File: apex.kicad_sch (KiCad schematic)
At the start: 15 parts, among them J1 USB_C_Receptacle_USB2.0_16P, U1 AP7363-33D-13, U2 USBLC6-2P6

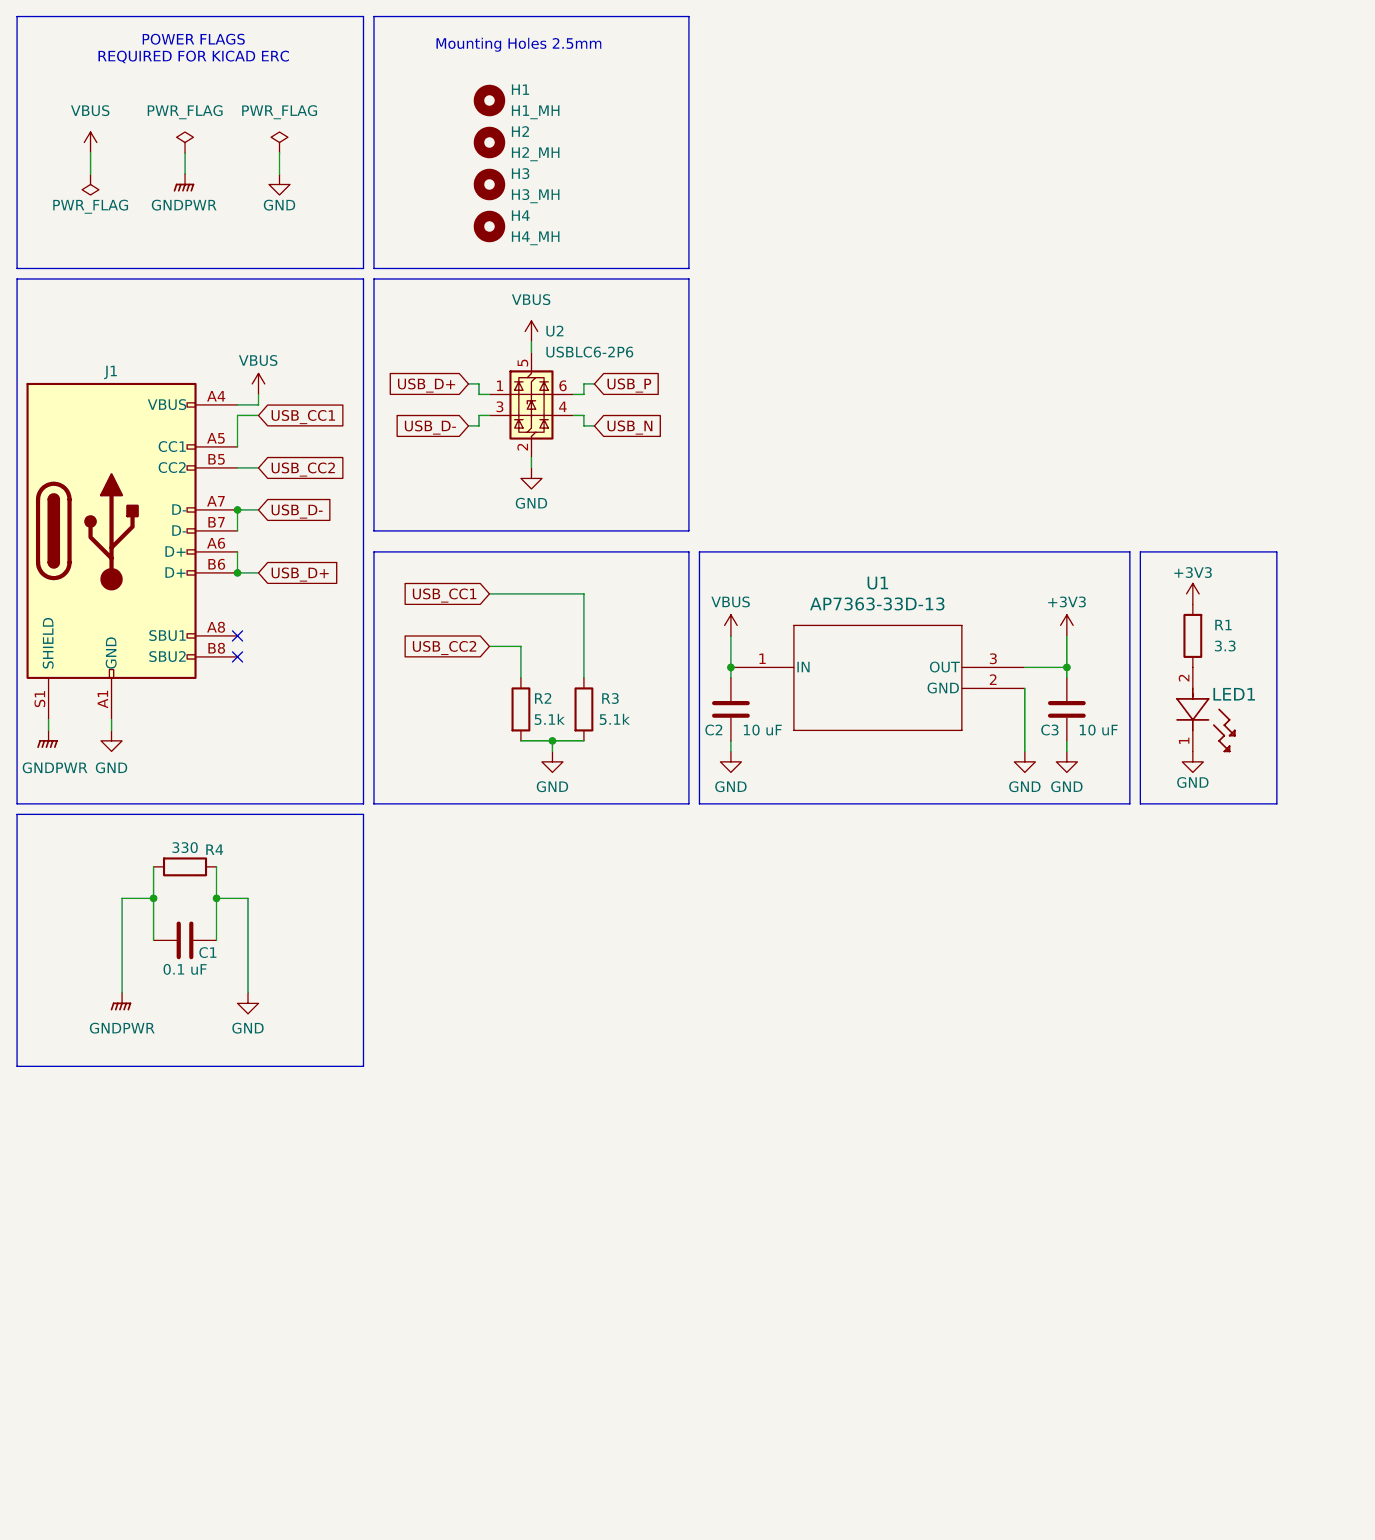
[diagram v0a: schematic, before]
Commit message: re-added symbols
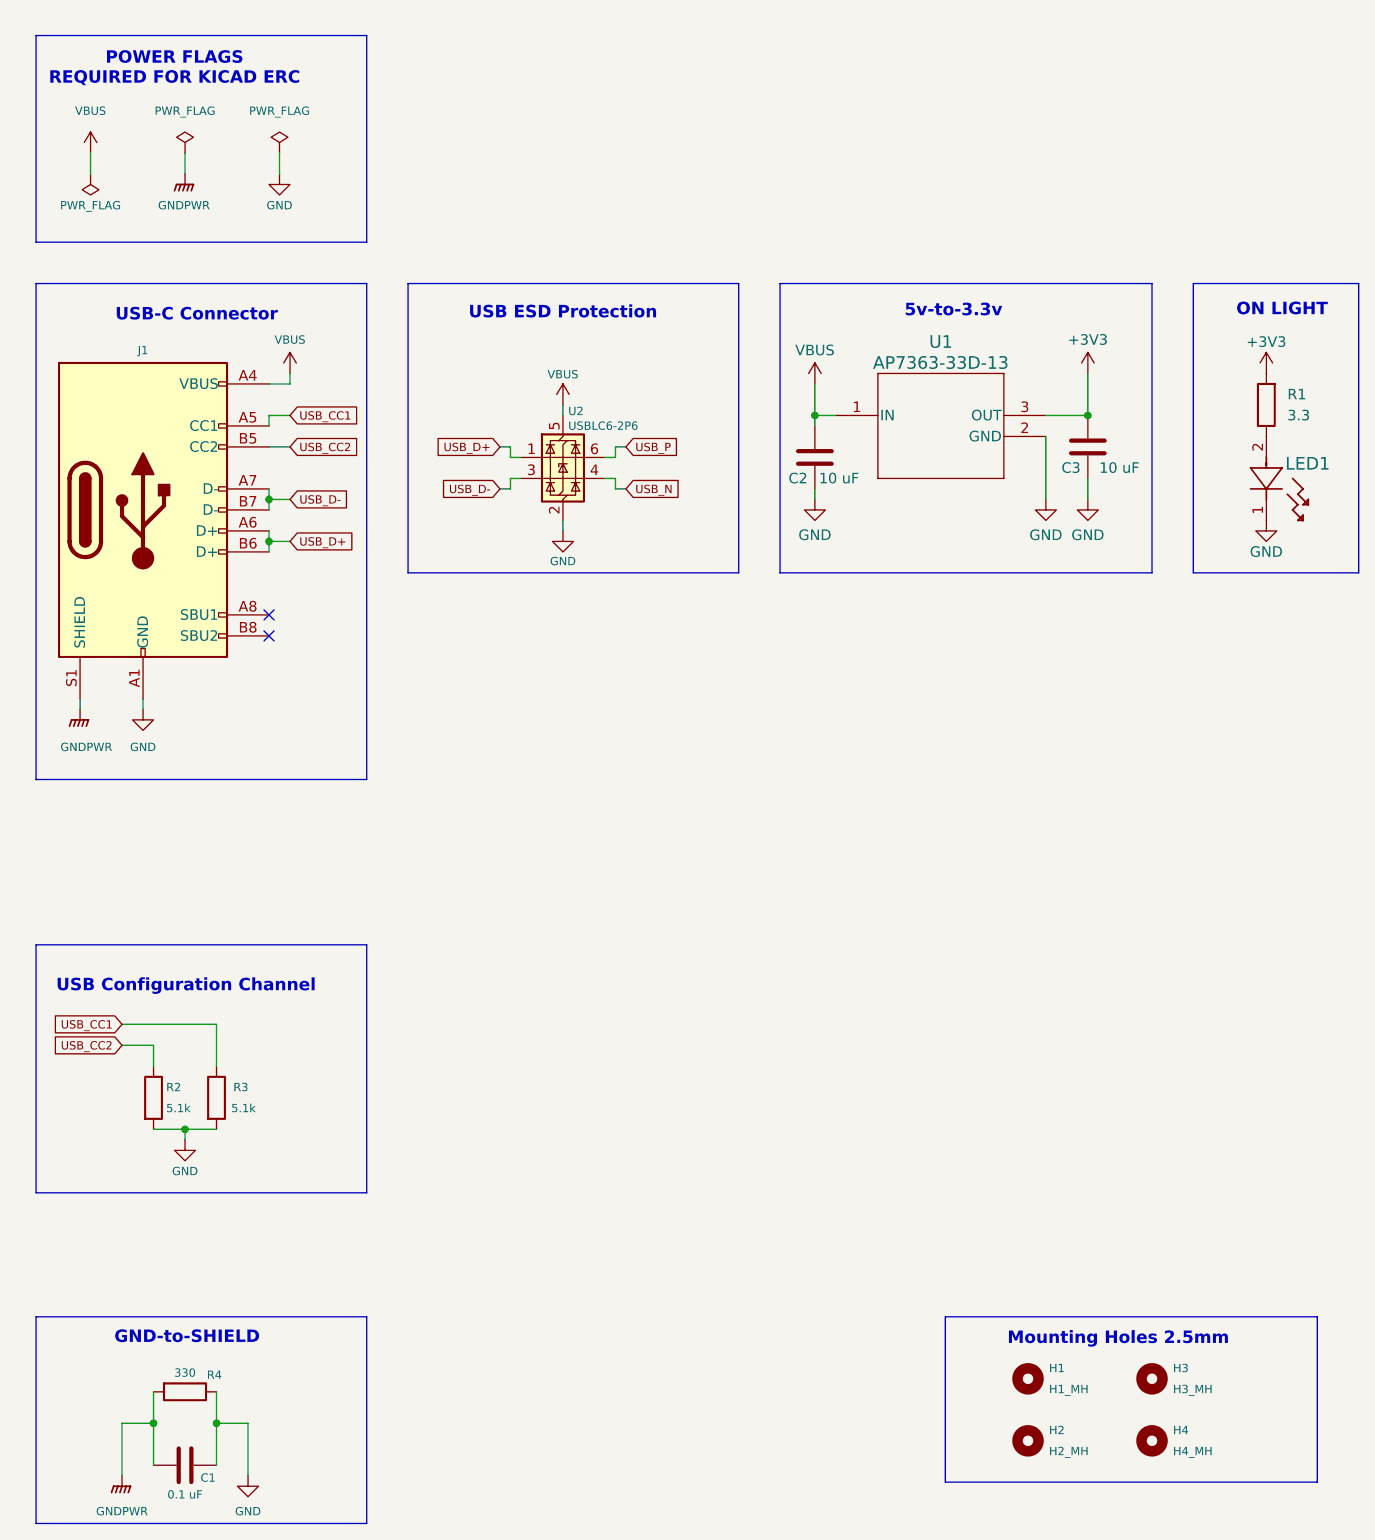
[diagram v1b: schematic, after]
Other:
- note added: "5v-to-3.3v"
- note added: "GND-to-SHIELD"
- note added: "ON LIGHT"
- note added: "USB Configuration Channel"
- note added: "USB ESD Protection"
- note added: "USB-C Connector"
- moved on the sheet: C1, C2, C3, H1, H2, H3, H4, J1, LED1, R1, R2, R3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
